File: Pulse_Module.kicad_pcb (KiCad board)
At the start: 2 copper layers, 100.2 x 70.9 mm, 67 parts, among them CON1 AVR-ISP-10, CON2 AVR-JTAG-10, CON3 BARREL_JACK, IC1 ATMEGA1280-A, P1 CONN_02X20, P2 USB_OTG, P3 CONN_01X03, P4 CONN_01X03, SW1 SW_PUSH, U1 74HCT541_PWR, U2 PL2303, U3 AMS1117, U6 WS2812, U7 WS2812, U8 WS2812, X1 CRYSTAL, Y1 CRYSTAL

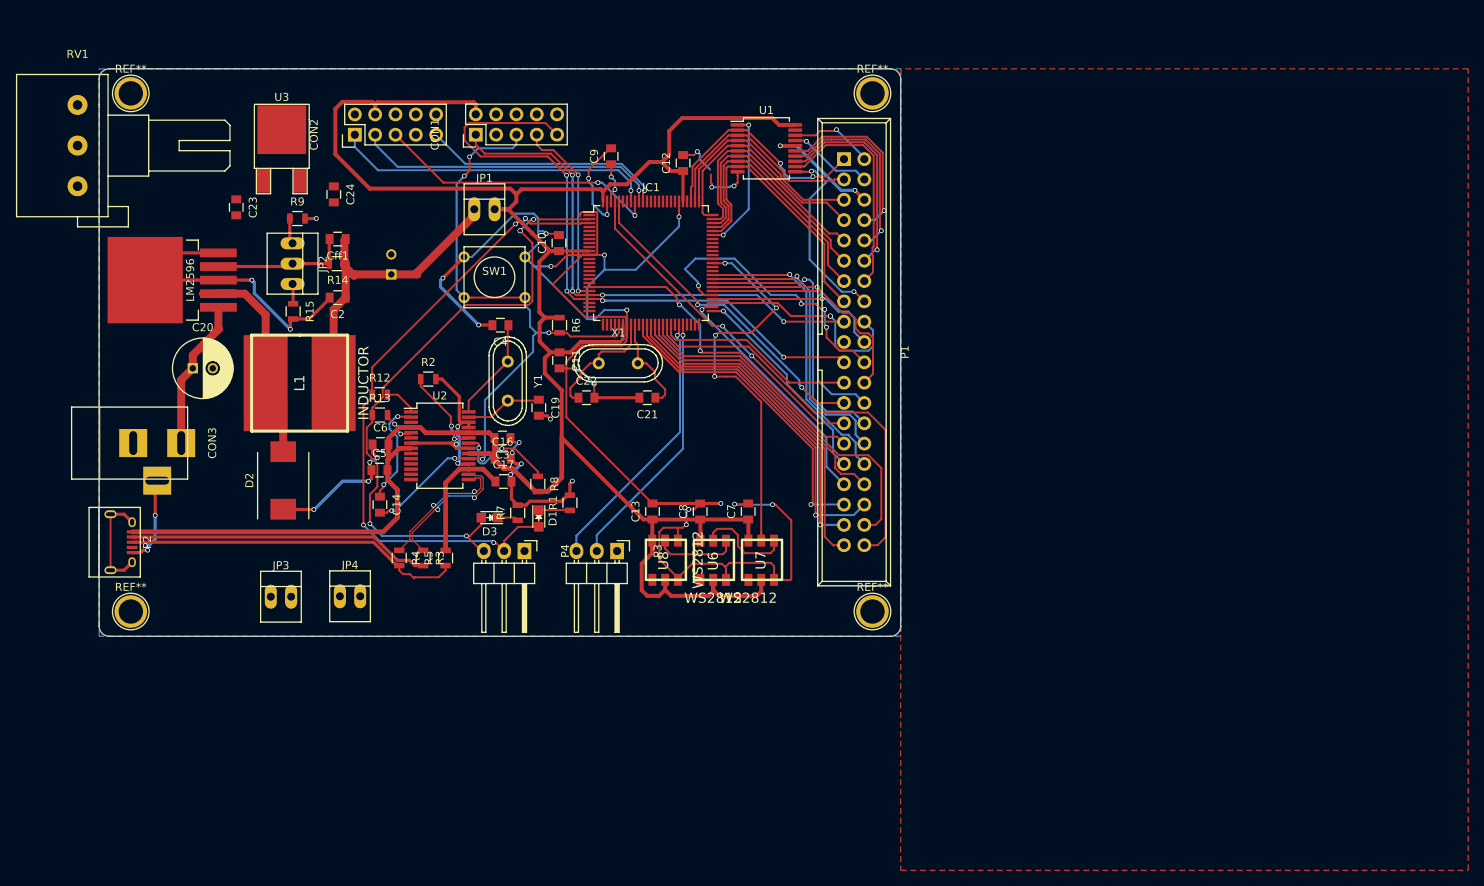
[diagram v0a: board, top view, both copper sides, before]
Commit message: Последние изменения
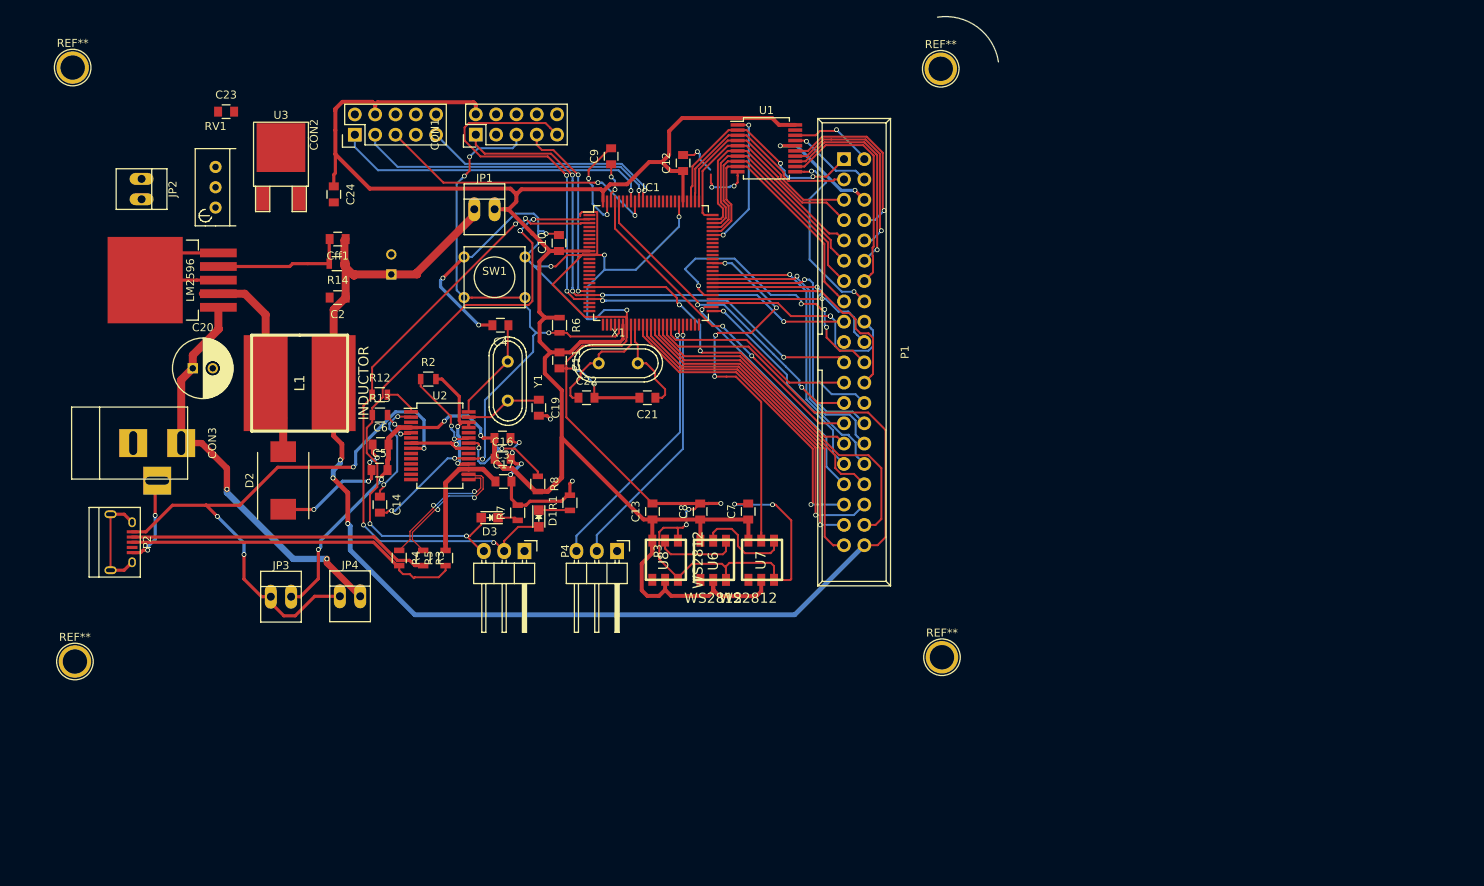
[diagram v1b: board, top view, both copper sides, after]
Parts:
- removed R15: 1k, Resistors_SMD:R_0805
- removed R9: R, Resistors_SMD:R_0805
- C23: value C -> 10uF
- JP2: footprint Connect:PINHEAD1-3 -> Connect:PINHEAD1-2
- RV1: footprint Potentiometers:Potentiometer_Alps-RK163-single_15mm -> Potentiometers:Potentiometer_Bourns_3296W_3-8Zoll_Inline_ScrewUp
- moved JP2 21.0 mm to (108.0, 93.9)
- moved RV1 17.5 mm to (117.3, 96.2)
- moved C23 12.0 mm to (118.6, 84.2), turned to 0 degrees
- moved REF** 10.4 mm to (208.1, 152.4)
- moved REF** 9.37 mm to (99.7, 152.9)
- moved REF** 9.07 mm to (207.9, 78.8)
- moved REF** 7.95 mm to (99.4, 78.7)
- moved U3 2.24 mm to (125.5, 95.0)
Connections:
- net /Sheet56DEE0DD/34 renamed /Sheet56DEE0DD/А16
- net /Sheet56DEE0DD/35 renamed /Sheet56DEE0DD/Dout1
- net /Sheet56DEE0DD/37 renamed /Sheet56DEE0DD/CLK1
- net /Sheet56DEE0DD/39 renamed /Sheet56DEE0DD/CS1
- P1 pad 40: USB_IN -> /Sheet56DEE0DD/Vcc
- U2 pad 20: VCC -> USB_IN
- U2 pad 24: VCC -> USB_IN
- U2 pad 8: VCC -> USB_IN
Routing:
- net (no net): track 2.51 -> 236.6 mm
- net /Sheet56DEE0DD/Vcc: track 42.0 -> 184.1 mm, vias 0 -> 3
- net Net-(IC1-Pad42): track 48.4 -> 1.30 mm
- net USB_IN: track 33.0 -> 75.8 mm, vias 0 -> 4
- net /Sheet56D88A8D/Vin: track 19.0 -> 51.4 mm, vias 0 -> 2
- net GND: track 365.0 -> 344.2 mm, vias 37 -> 34
- net +5V: track 267.5 -> 286.9 mm, vias 0 -> 4
- net VCC: track 8.20 -> 0.00 mm
- net Net-(JP2-Pad1): track 2.78 -> 0.00 mm
- net /Sheet56D88A8D/FB: track 14.7 -> 17.1 mm
- net Net-(C23-Pad1): track 2.41 -> 0.00 mm
- removed copper zone on B.Cu, net GND
- removed copper zone on F.Cu, net GND
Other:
- board size 100.2 x 70.9 mm -> 7.6 x 5.7 mm
